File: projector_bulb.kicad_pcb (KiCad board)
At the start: 2 copper layers, 85.7 x 85.7 mm, 45 parts, among them J1 to_upright_+, J2 to_upright_-, J3 to_base, J4 Conn_02x02_Odd_Even, J5 Conn_02x02_Odd_Even, U1 PAM2863, U2 AP7381-33Y

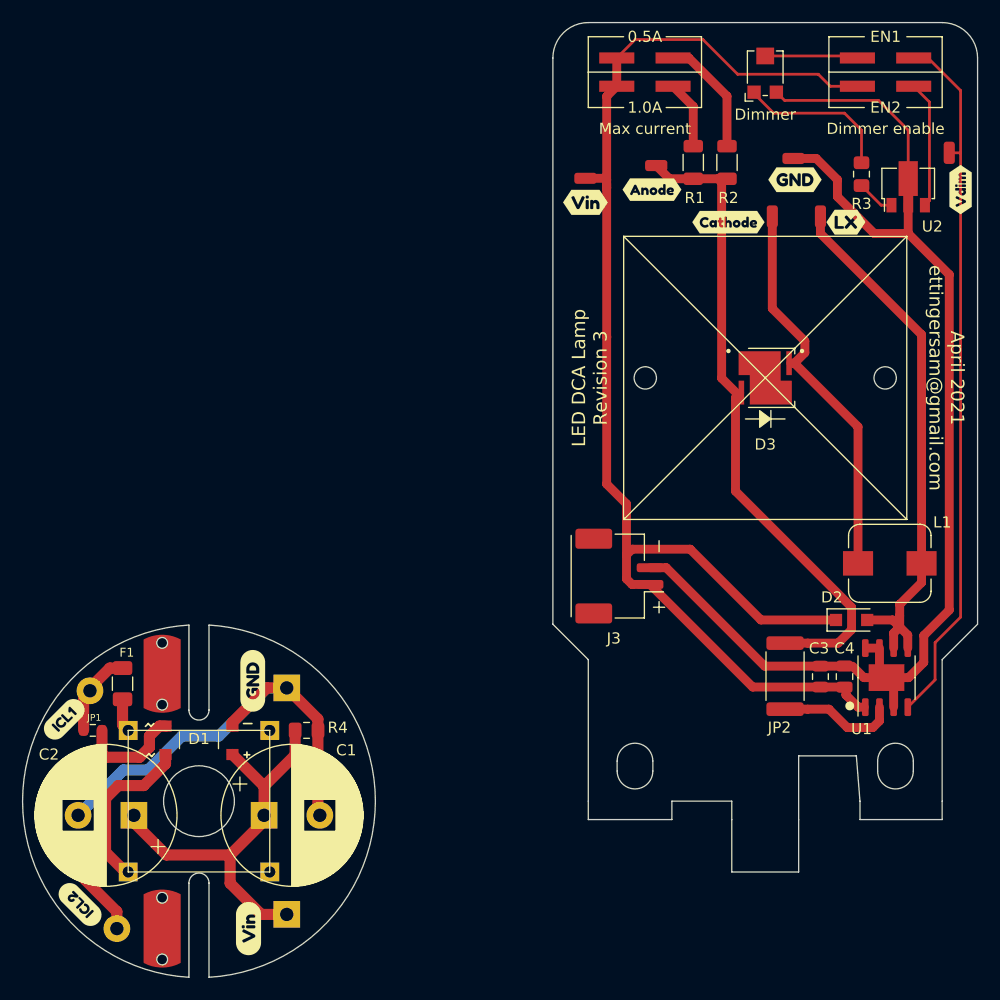
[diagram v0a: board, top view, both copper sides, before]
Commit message: Added fillets after much blood sweat and tears
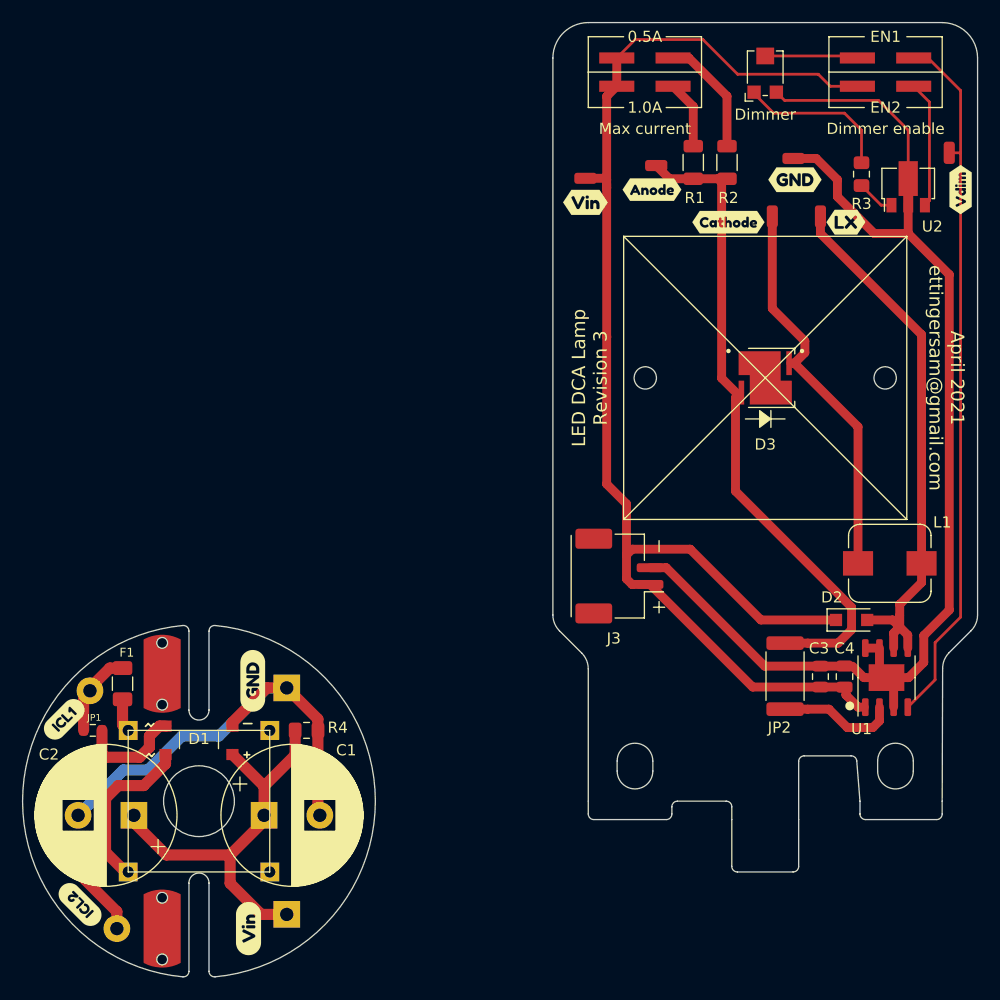
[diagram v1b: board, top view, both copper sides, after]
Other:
- board size 85.7 x 85.7 mm -> 85.7 x 85.6 mm
